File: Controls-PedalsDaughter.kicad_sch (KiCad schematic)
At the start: 21 parts, among them J2 Accel Pos. Sensor, J3 PeripheralCANConnector, J4 Conn_01x02, J5 PeripheralCANConnector, U1 RI3-1205S, U2 PeripheralSOM

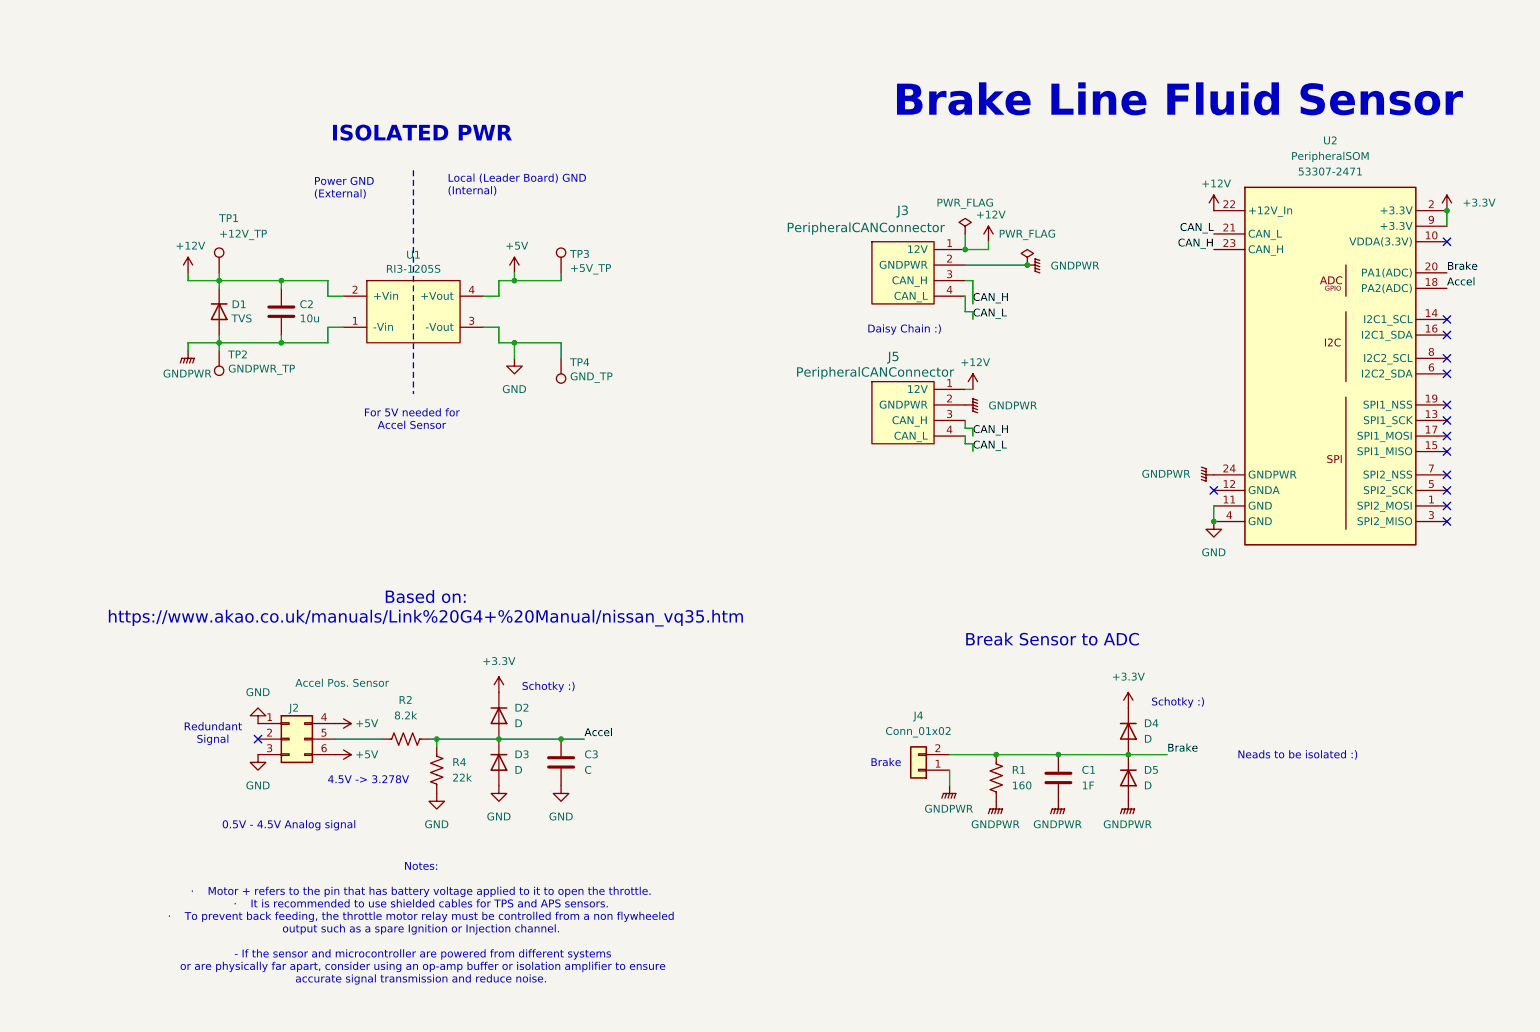
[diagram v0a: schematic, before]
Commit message: Added isolation n stuff
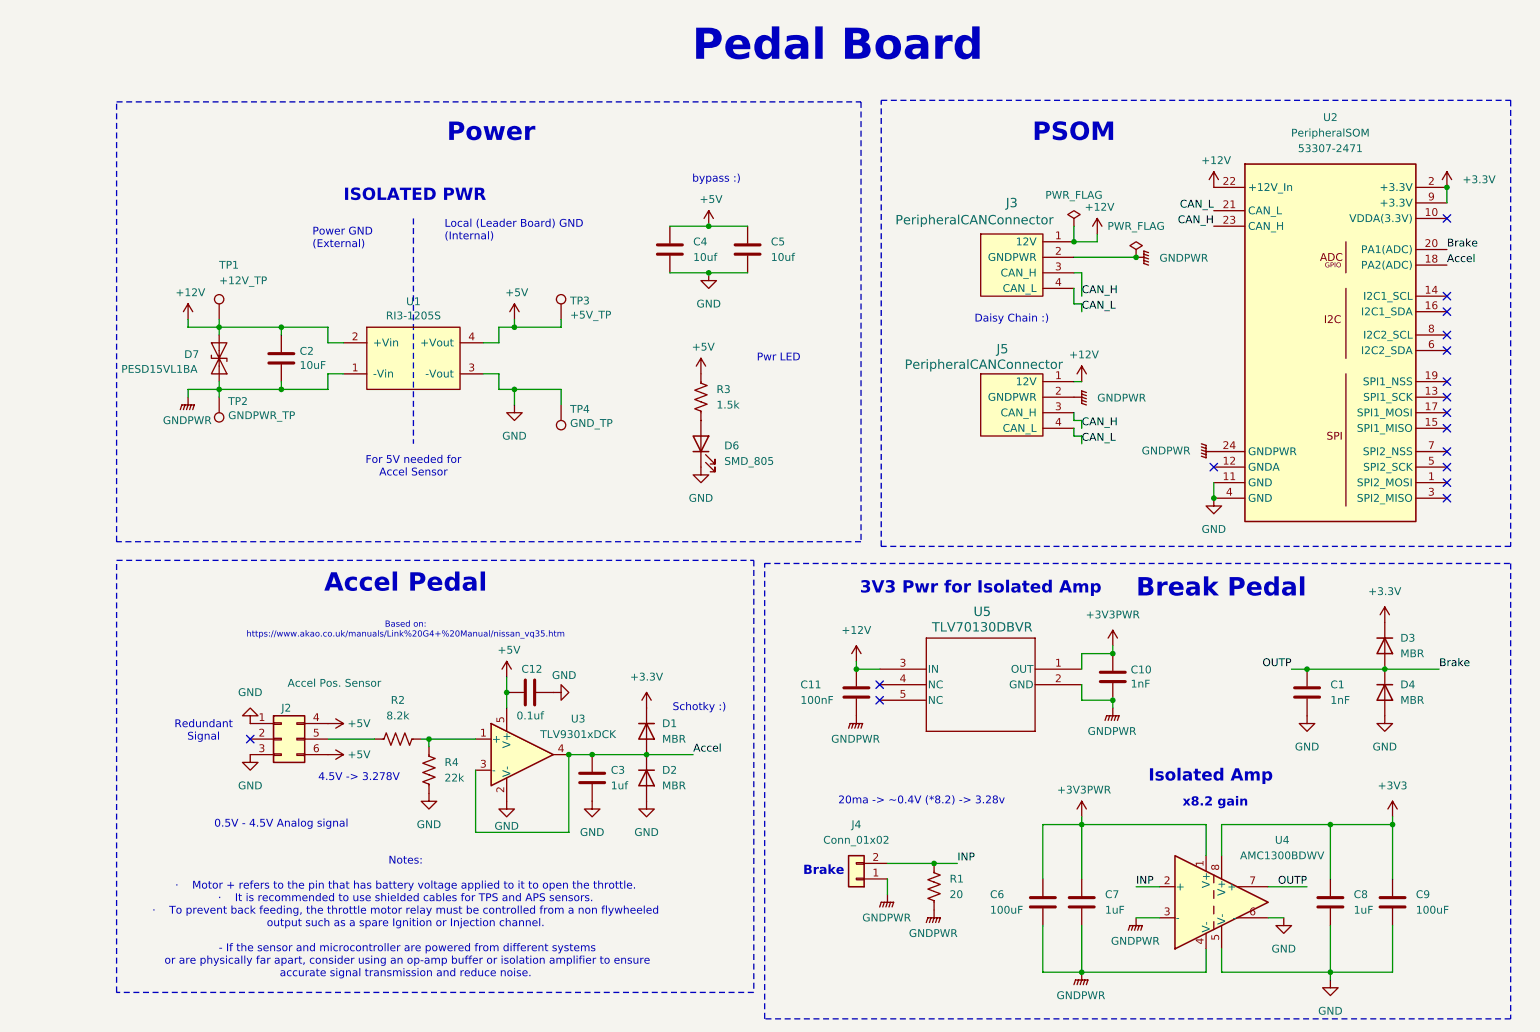
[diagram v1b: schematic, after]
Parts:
- removed D5: D, symbol Device:D
- added C10: 1nF, Capacitor_SMD:C_0805_2012Metric, symbol Device:C
- added C11: 100nF, Capacitor_SMD:C_0805_2012Metric, symbol Device:C
- added C12: 0.1uf, symbol Device:C
- added C4, C5: 10uf, symbol Device:C
- added C6, C9: 100uF, symbol Device:C
- added C7, C8: 1uF, symbol Device:C
- added D6: SMD_805, symbol Device:LED
- added D7: PESD15VL1BA, Diode_SMD:D_SOD-323, symbol Diode:SD12_SOD323
- added R3: 1.5k, symbol Device:R_US
- added U3: TLV9301xDCK, Package_TO_SOT_SMD:SOT-353_SC-70-5, symbol Amplifier_Operational:TLV9301xDCK
- added U4: AMC1300BDWV, Package_SO:SOIC-8_7.5x5.85mm_P1.27mm, symbol Amplifier_Difference:AMC1300BDWV
- added U5: TLV70130DBVR, UTSVT_Power:TLV70130DBVR, symbol 2025-01-18_20-51-31:TLV70130DBVR
- C1: value 1F -> 1nF
- C2: value 10u -> 10uF
- C3: value C -> 1uf
- D1: value TVS -> MBR; footprint Diode_SMD:D_SOD-323 -> (none); P/N (none) -> MBR0520LT1G
- D2, D3, D4: value D -> MBR; P/N (none) -> MBR0520LT1G
- R1: value 160 -> 20
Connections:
- net +12V: now also C11.1, D7.2 (A2), U5.3 (IN); no longer D1.1 (K)
- net +3.3V: now also D1.1 (K), D3.1 (K); no longer D2.1 (K), D4.1 (K)
- net +5V: now also C12.2, C4.1, C5.1, R3.1, U3.5 (V+)
- net Accel: now also D1.2 (A), D2.1 (K), U3.3 (-), U3.4; no longer D2.2 (A), D3.1 (K), R2.1, R4.1
- net Brake: now also D3.2 (A), D4.1 (K), U4.7 (+); no longer D4.2 (A), J4.2 (Pin_2), R1.1
- net GND: now also C1.2, D2.2 (A), D4.2 (A), C12.1, C4.2, C5.2, C8.2, C9.2, D6.1 (K), U3.2 (V-), U4.5 (V-), U4.6 (-); no longer D3.2 (A)
- net GNDPWR: now also C10.2, C11.2, C6.2, C7.2, D7.1 (A1), U4.3 (-), U4.4 (V-), U5.2 (GND); no longer C1.2, D1.2 (A)
- new net: R2.1, R4.1, U3.1 (+)
- new net: D6.2 (A), R3.2
- new net +3V3: C8.1, C9.1, U4.8 (V+)
- new net +3V3PWR: C10.1, C6.1, C7.1, U4.1 (V+), U5.1 (OUT)
- new net INP: J4.2 (Pin_2), R1.1, U4.2 (+)
- no-connect marks 15 -> 17
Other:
- note added: "20ma -> ~0.4V (*8.2) -> 3.28v"
- note added: "3V3 Pwr for Isolated Amp"
- note added: "Accel Pedal"
- note added: "Break Pedal"
- note added: "Isolated Amp"
- note added: "PSOM"
- note added: "Pedal Board"
- note added: "Power"
- note added: "Pwr LED"
- note added: "bypass :)"
- note added: "x8.2 gain"
- note removed: "Brake Line Fluid Sensor"
- note removed: "Break Sensor to ADC"
- note removed: "Neads to be isolated :)"
- moved on the sheet: C2, J2, J3, J4, J5, R1, R2, R4, TP1, TP2, TP3, TP4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
